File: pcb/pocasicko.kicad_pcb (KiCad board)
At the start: 2 copper layers, 100 x 88 mm, 61 parts, among them J1 SMA, J2 Header_SMD_1x05, J3 FPC24, J4 Header_SMD_1x03, Q1 AO3400A, SW1 SW_Push, SW2 A, SW3 B, SW4 C, SW5 D, U1 CMWX1ZZABZ-091, U2 BME680, U3 MP28200, U4 LM66100

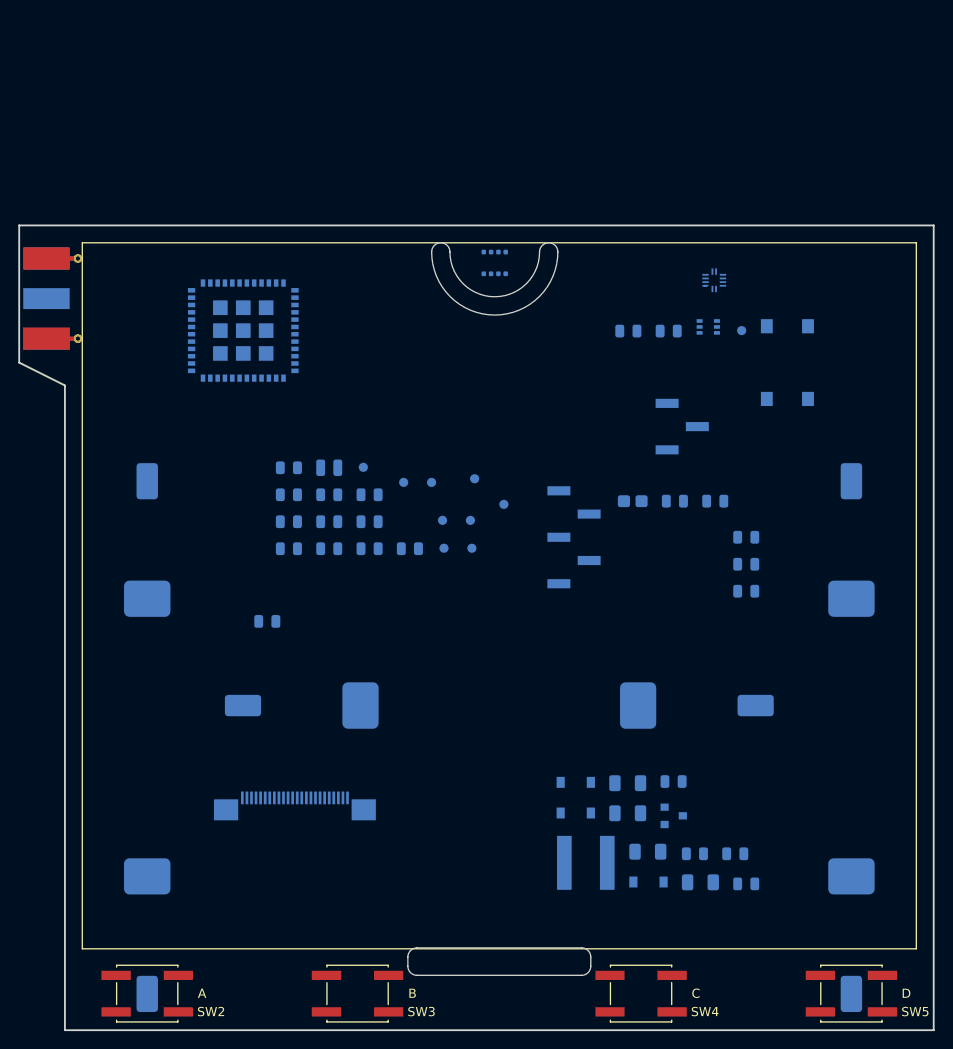
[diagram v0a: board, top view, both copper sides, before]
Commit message: Routing progress
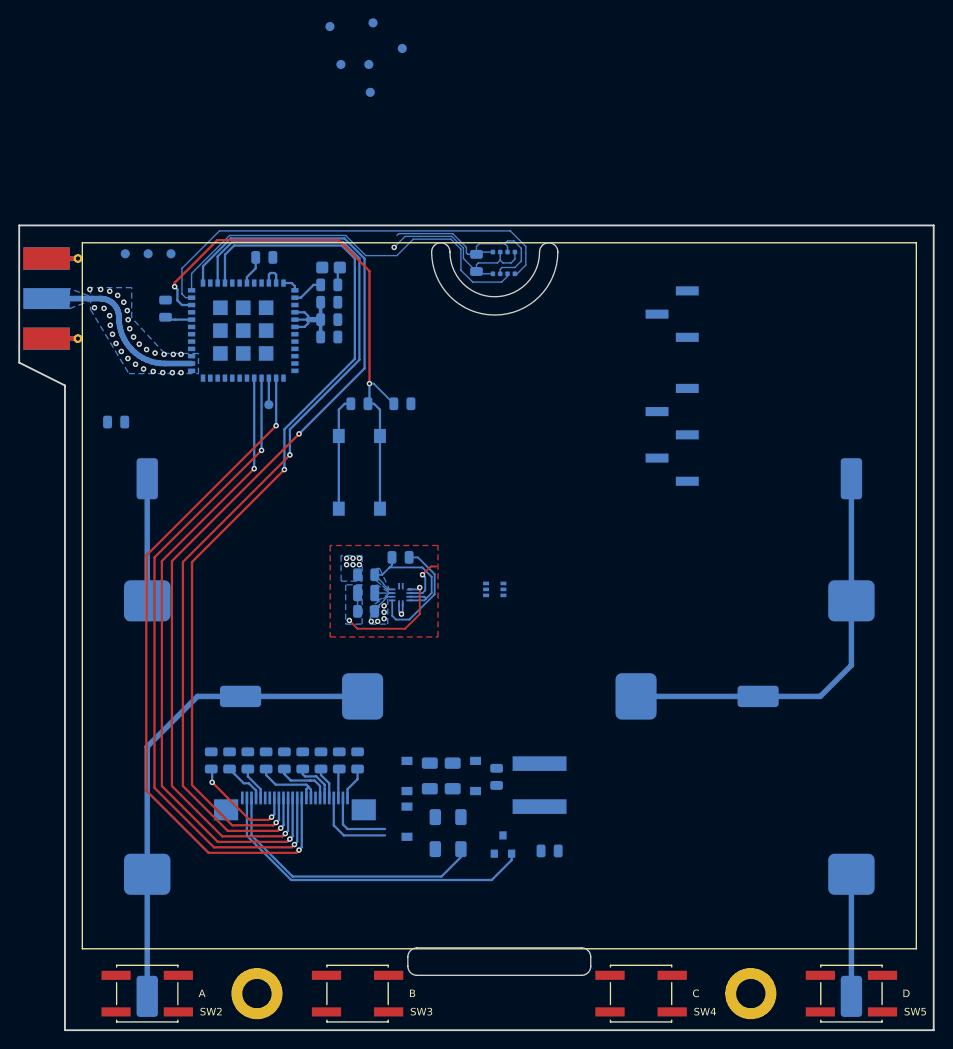
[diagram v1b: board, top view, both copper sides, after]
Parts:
- added C20: 1uF, Capacitor_SMD:C_0805_2012Metric, B.Cu at (116.0, 59.1)
- added H1: M3_Hole, MountingHole:MountingHole_3.2mm_M3_DIN965_Pad, F.Cu at (126.0, 134.0)
- added H2: M3_Hole, MountingHole:MountingHole_3.2mm_M3_DIN965_Pad, F.Cu at (180.0, 134.0)
- added REF**: KiCad-Logo_5mm_SilkScreen, Symbol:KiCad-Logo_5mm_SilkScreen, B.Cu at (187.9, 58.6)
- moved R7 56.9 mm to (110.6, 71.5)
- moved R1 56.1 mm to (126.8, 53.5)
- moved C3 55.5 mm to (133.9, 58.4), turned to 180 degrees
- moved C19 54.2 mm to (127.0, 108.5), turned to -90 degrees
- moved R2 53.3 mm to (133.9, 56.5)
- moved C5 52.9 mm to (133.9, 60.3), turned to 180 degrees
- moved TP10 52.3 mm to (127.3, 69.6)
- moved TP6 51.1 mm to (138.7, 27.9)
- moved TP8 51.1 mm to (138.2, 32.4)
- moved TP9 51.1 mm to (141.9, 30.6)
- moved TP4 51.1 mm to (135.2, 32.4)
- moved TP5 51.1 mm to (138.4, 35.5)
- moved TP7 51.1 mm to (134.0, 28.2)
- moved R6 50.6 mm to (121.0, 108.5), turned to 90 degrees
- moved U3 48.6 mm to (141.7, 90.4), turned to 180 degrees
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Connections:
- C12 pad 2: +2V5 -> /VPP
- U2 pad 2: +3V3 -> +2V5
- U3 pad 1: Net-(L1-Pad1) -> +2V5
- U3 pad 9: +2V5 -> Net-(L1-Pad1)
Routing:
- net /D/C#: track 0.00 -> 106.9 mm, vias 0 -> 2
- net /RES#: track 0.00 -> 101.8 mm, vias 0 -> 2
- net /BUSY: track 0.00 -> 97.2 mm, vias 0 -> 2
- net /SDI: track 0.00 -> 76.4 mm, vias 0 -> 2
- net /SCLK: track 0.00 -> 73.0 mm, vias 0 -> 2
- net /CS#: track 0.00 -> 70.1 mm, vias 0 -> 2
- net +2V5: track 0.00 -> 60.5 mm, vias 0 -> 2
- net /~MCU_RESET: track 0.00 -> 59.0 mm, vias 0 -> 2
- net Net-(BT2-Pad1): track 0.00 -> 53.1 mm
- net GND: track 0.00 -> 51.7 mm, vias 0 -> 42
- net /BME680_SCL: track 0.00 -> 47.6 mm
- net Net-(BT1-Pad1): track 0.00 -> 45.4 mm
- net /BME680_SDA: track 0.00 -> 43.6 mm
- net /GDR: track 0.00 -> 36.7 mm
- net /RESE: track 0.00 -> 30.6 mm
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- added copper zone on B.Cu, net +2V5
- added copper zone on B.Cu, net /BATT_VOLTAGE
- added copper zone on B.Cu, net GND
- added copper zone on F.Cu, net GND
- added copper zone on B.Cu, net Net-(J1-Pad1)
- added copper zone on B.Cu, net Net-(L1-Pad1)
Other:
- net class Default: clearance 0.2 -> 0.127
- rule pad_to_mask_clearance: 0.051 -> 0
- rule solder_mask_min_width: 0.25 -> 0.12
- rule trace_clearance: 0.2 -> 0.127
- rule trace_min: 0.2 -> 0.127
- rule via_min_size: 0.4 -> 0.6
- board text added: "GND"
- board text added: "NRST"
- board text added: "RX"
- board text added: "SWCLK"
- board text added: "SWDIO"
- board text added: "TX"
- board text added: "VDD"
